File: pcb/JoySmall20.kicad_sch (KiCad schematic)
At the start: 57 parts, among them J1 AudioJack4, SW1 SW_Push, SW10 SW_Push, SW11 SW_Push, SW12 SW_Push, SW13 SW_Push, SW14 SW_Push, SW15 SW_Push, SW16 SW_Push, SW17 SW_Push, SW18 SW_Push, SW19 SW_Push, SW2 SW_Push, SW20 SW_Push, SW3 SW_Push, SW4 SW_Push, SW5 SW_Push, SW6 SW_Push, SW7 SW_Push, SW8 SW_Push, SW9 SW_Push

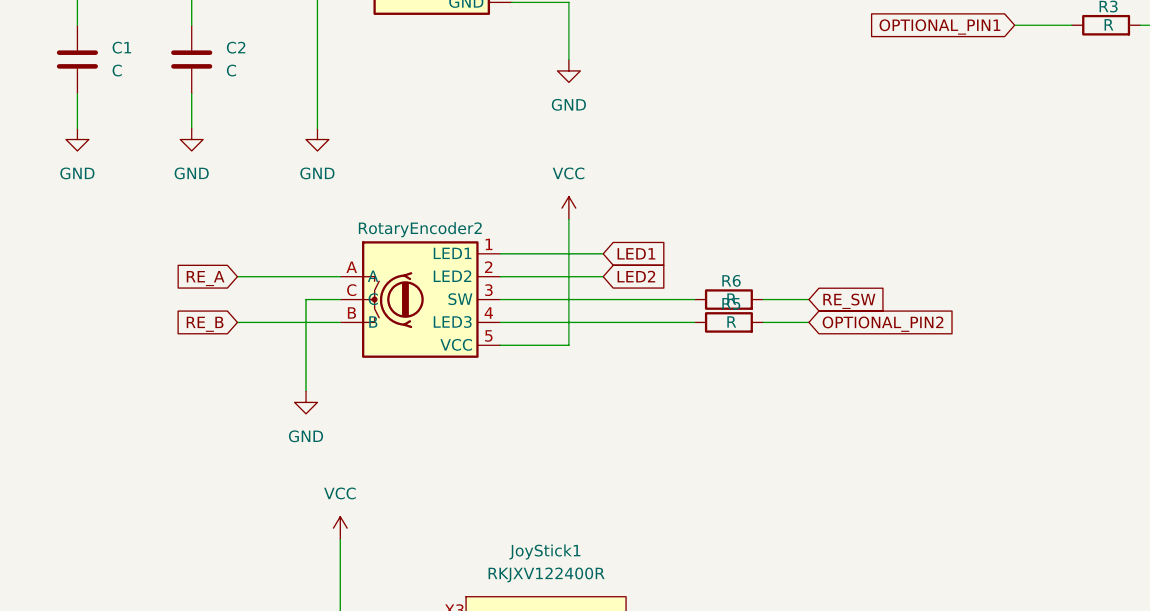
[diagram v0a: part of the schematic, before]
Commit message: feat: readmeを追加
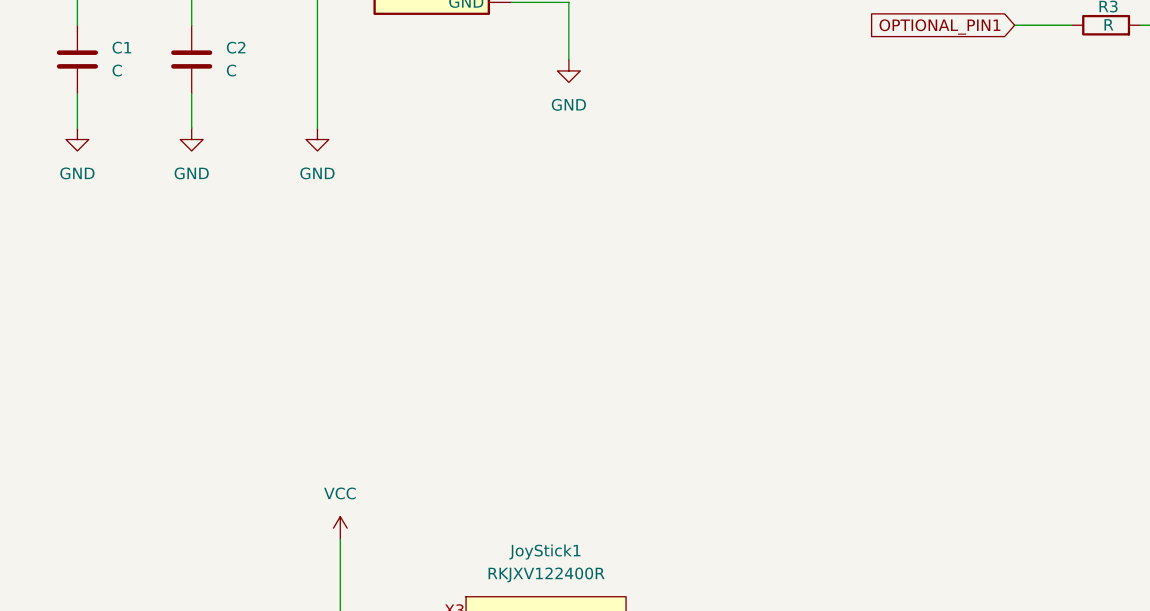
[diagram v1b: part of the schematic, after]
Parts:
- removed R5, R6: R, Resistor_THT:R_Axial_DIN0207_L6.3mm_D2.5mm_P7.62mm_Horizontal, symbol Device:R
- removed RotaryEncoder2: ~, xxx_original:RotaryEncoder_with_5pin, symbol xxx_original:RotaryEncoder_Switch_3LED
